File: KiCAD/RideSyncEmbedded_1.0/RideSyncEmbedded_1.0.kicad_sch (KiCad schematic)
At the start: 29 parts, among them IC1 LTC3108, IC2 LTC3108, T1 PA0185NL, U2 LT6106, U3 LT6106, U6 SiP32431DR3, U7 SiP32431DR3

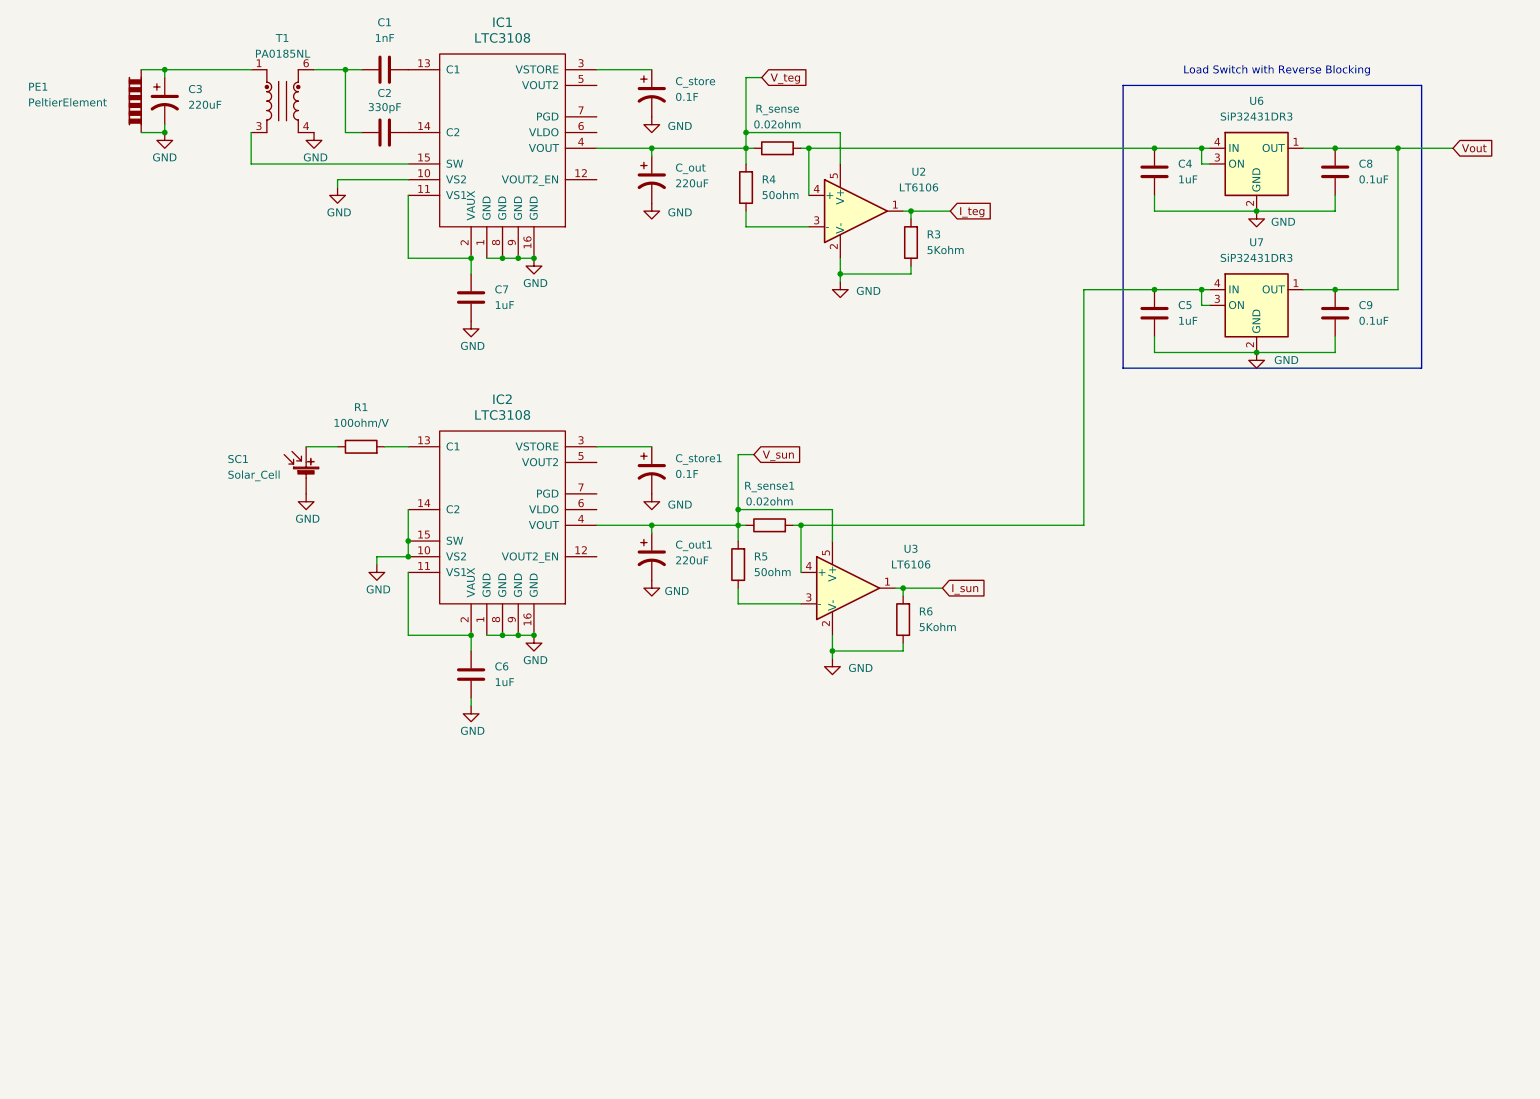
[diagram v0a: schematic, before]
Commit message: 0.1 update
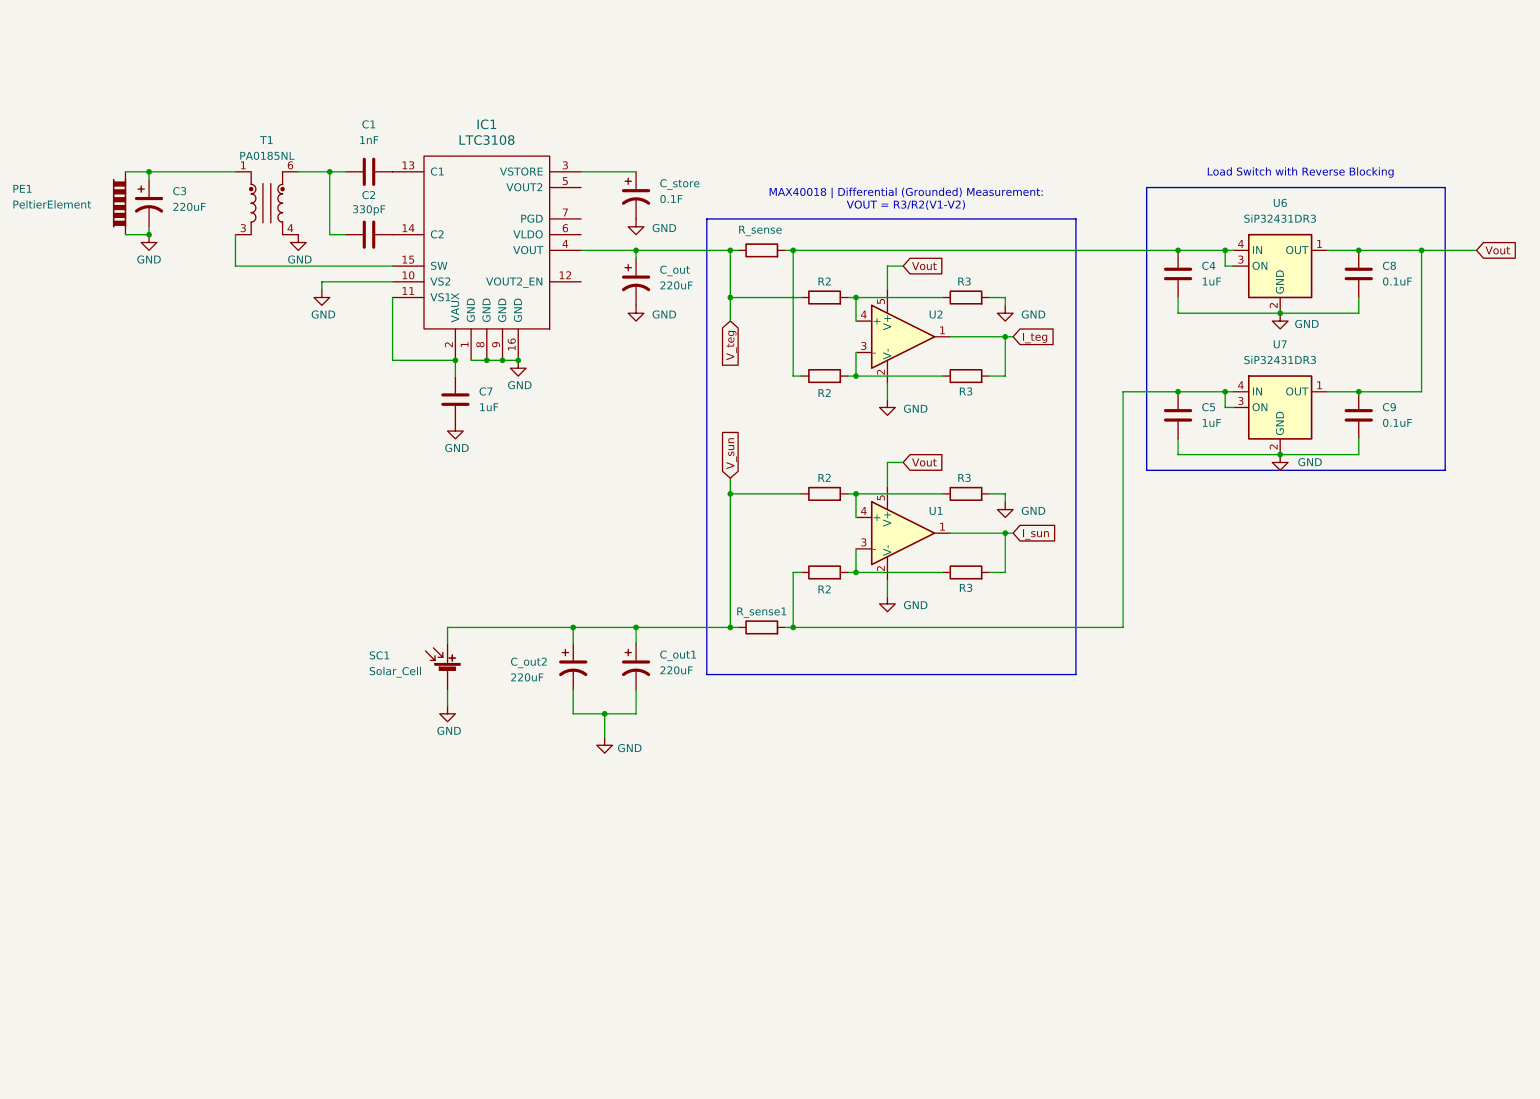
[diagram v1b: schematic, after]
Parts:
- removed C6: 1uF, symbol Device:C
- removed C_store1: 0.1F, symbol Device:C_Polarized_US
- removed IC2: LTC3108, symbol ltc3108-cache:LTC3108
- removed R1: 100ohm/V, symbol Device:R
- removed R3, R6: 5Kohm, symbol Device:R
- removed R4, R5: 50ohm, symbol Device:R
- removed U3: LT6106, Package_TO_SOT_SMD:SOT-23-5, symbol Amplifier_Current:LT6106
- added C_out2: 220uF, symbol Device:C_Polarized_US
- added R2 (x4), R3 (x4): R, symbol Device:R
- added U1: LT6106, Package_TO_SOT_SMD:SOT-23-5, symbol Amplifier_Current:LT6106
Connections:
- net GND: now also C_out2.2, R3.2, R3.2, U1.2 (V-)
- net I_sun: now also R3.2, U1.1
- net I_teg: now also R3.2
- net V_sun: now also SC1.1 (+), C_out2.1, R2.1
- net V_teg: now also R2.1; no longer U2.5 (V+)
- net Vout: now also U2.5 (V+), U1.5 (V+)
- net at U2.3 (-): now also R2.2, R3.1
- net at C4.1, R_sense.2, U6.3 (ON)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: now also R2.1; no longer U2.4 (+)
- net at C5.1, R_sense1.2, U7.3 (ON)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: now also R2.1
- new net: R2.2, R3.1, U2.4 (+)
- new net: R2.2, R3.1, U1.3 (-)
- new net: R2.2, R3.1, U1.4 (+)
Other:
- note added: "MAX40018 | Differential (Grounded) Measurement: VOUT = R3/R2(V1-V2)"
- moved on the sheet: C1, C2, C3, C4, C5, C7, C8, C9, C_out, C_out1, C_store, IC1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

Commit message: schema uodate
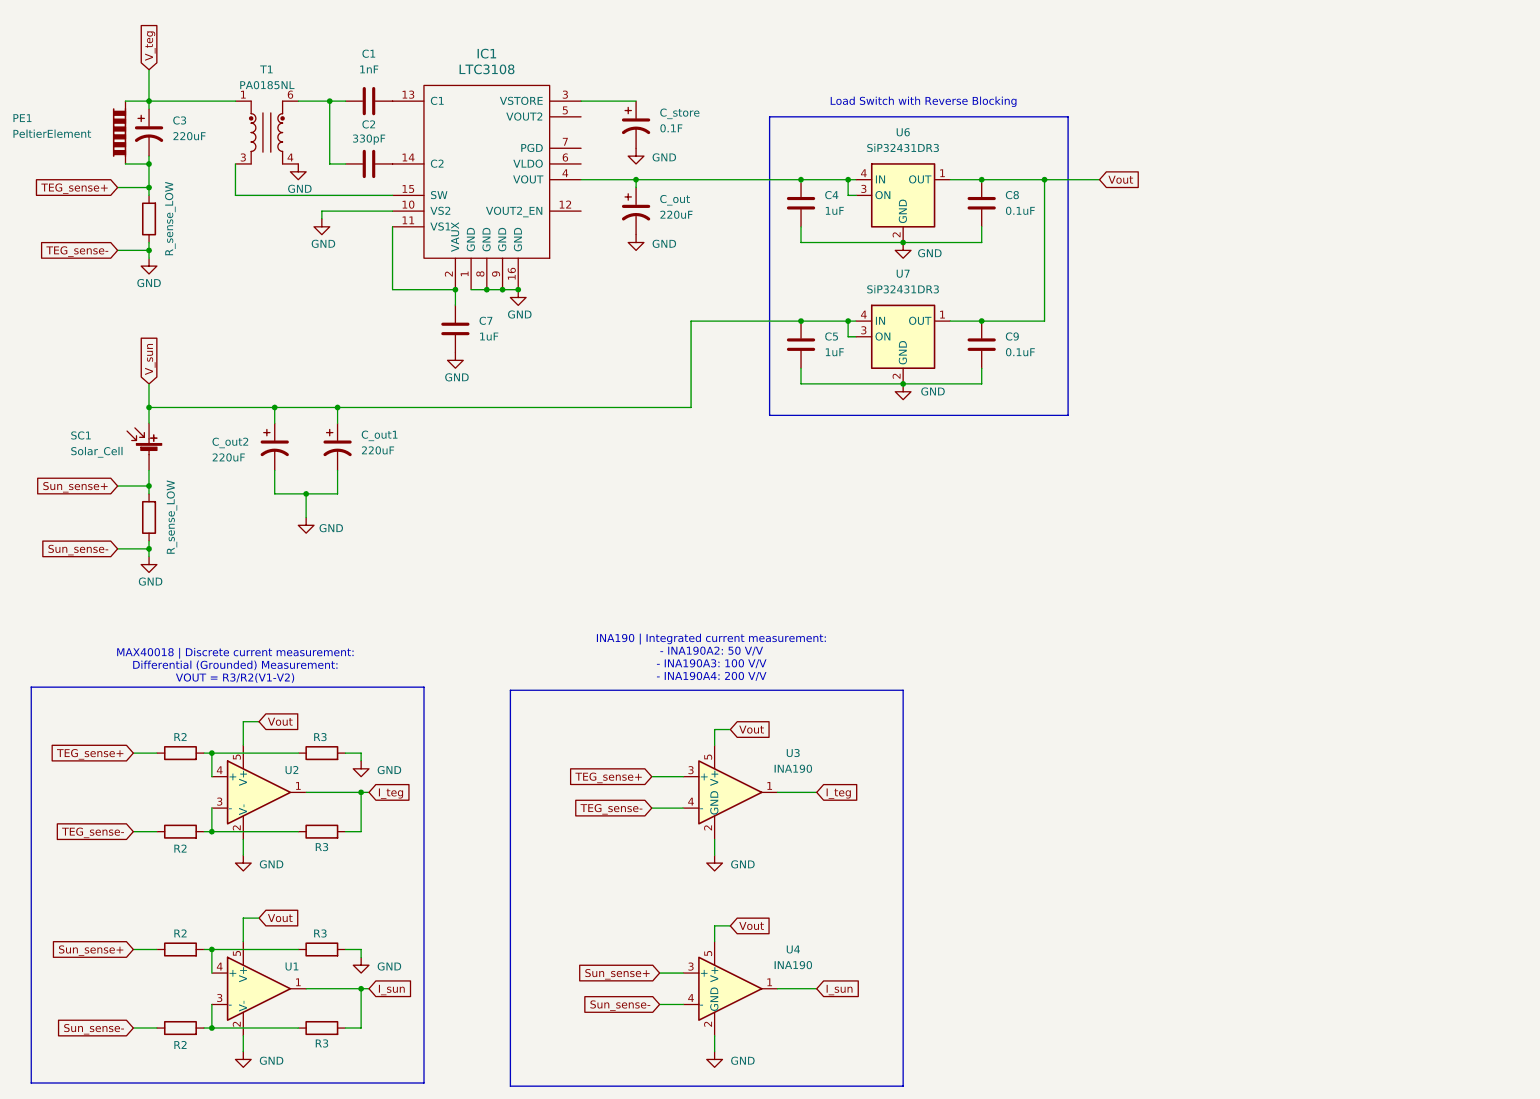
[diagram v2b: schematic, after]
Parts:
- removed R_sense, R_sense1: 0.02ohm, symbol Device:R
- added R_sense_LOW (x2): 0.02ohm, symbol Device:R
- added U3, U4: INA190, Package_TO_SOT_SMD:SOT-23, symbol Amplifier_Current1:INA190
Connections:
- net GND: now also R2.1, R2.1, R_sense_LOW.1, R_sense_LOW.1, U3.2 (GND), U3.4 (-), U4.2 (GND), U4.4 (-); no longer C3.2, PE1.1, SC1.2 (-)
- net I_sun: now also U4.1
- net I_teg: now also U3.1
- net V_sun: now also C5.1, U7.3 (ON), U7.4 (IN); no longer R2.1
- net V_teg: now also C3.1, PE1.2, T1.1; no longer C_out.1, IC1.4 (VOUT), R2.1
- net Vout: now also U3.5 (V+), U4.5 (V+)
- net at C4.1, U6.3 (ON), U6.4 (IN): now also C_out.1, IC1.4 (VOUT); no longer R2.1
- new net Sun_sense+: R2.1, R_sense_LOW.2, SC1.2 (-), U4.3 (+)
- new net TEG_sense+: C3.2, PE1.1, R2.1, R_sense_LOW.2, U3.3 (+)
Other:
- note added: "INA190 | Integrated current measurement: - INA190A2: 50 V/V - INA190A3: 100 V/V - INA190A4: 200 V/V"
- note added: "MAX40018 | Discrete current measurement: Differential (Grounded) Measurement: VOUT = R3/R2(V1-V2)"
- note removed: "MAX40018 | Differential (Grounded) Measurement: VOUT = R3/R2(V1-V2)"
- moved on the sheet: C1, C2, C3, C4, C5, C7, C8, C9, C_out, C_out1, C_out2, C_store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
